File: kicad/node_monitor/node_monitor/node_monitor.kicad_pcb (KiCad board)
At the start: 2 copper layers, 232.4 x 170.2 mm, 68 parts, among them J1 Conn_01x02_Male, J2 Conn_01x02_Male, J3 Conn_01x03_Male, J4 RJ45, J5 Conn_01x02_Male, J6 Conn_01x03_Male, J7 Conn_01x03_Male, J8 Conn_01x02_Male, SW1 SW_DIP_x06

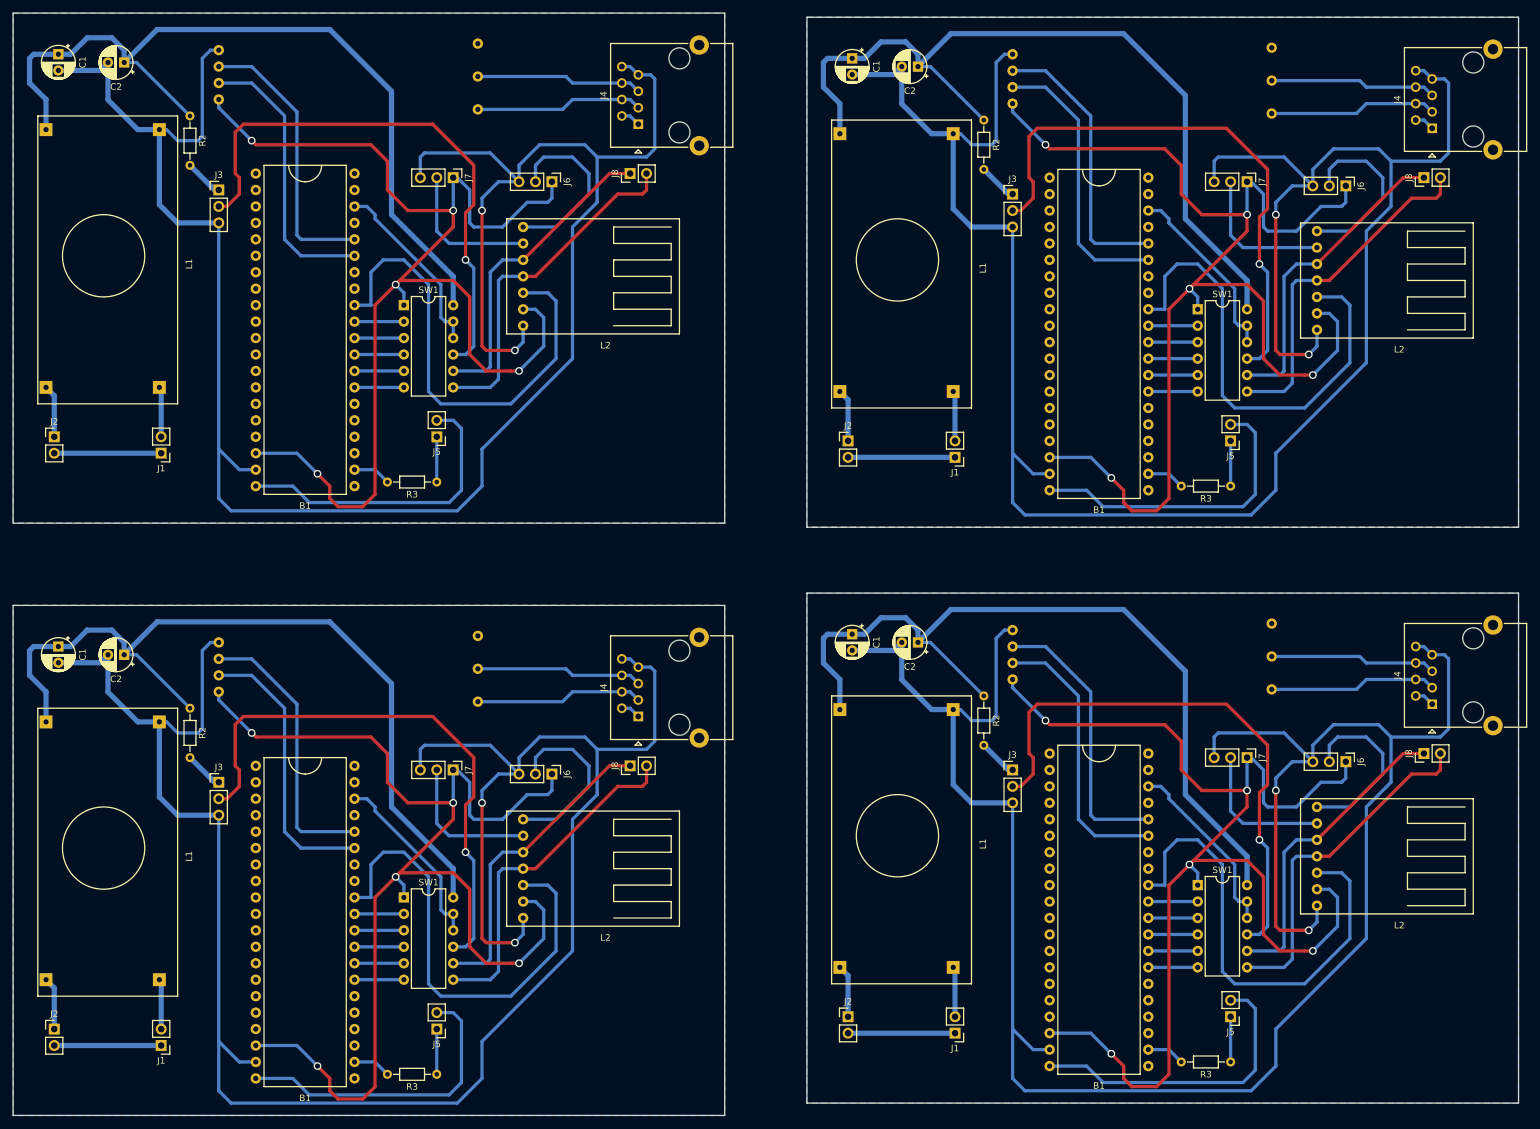
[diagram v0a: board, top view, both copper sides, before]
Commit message: 984
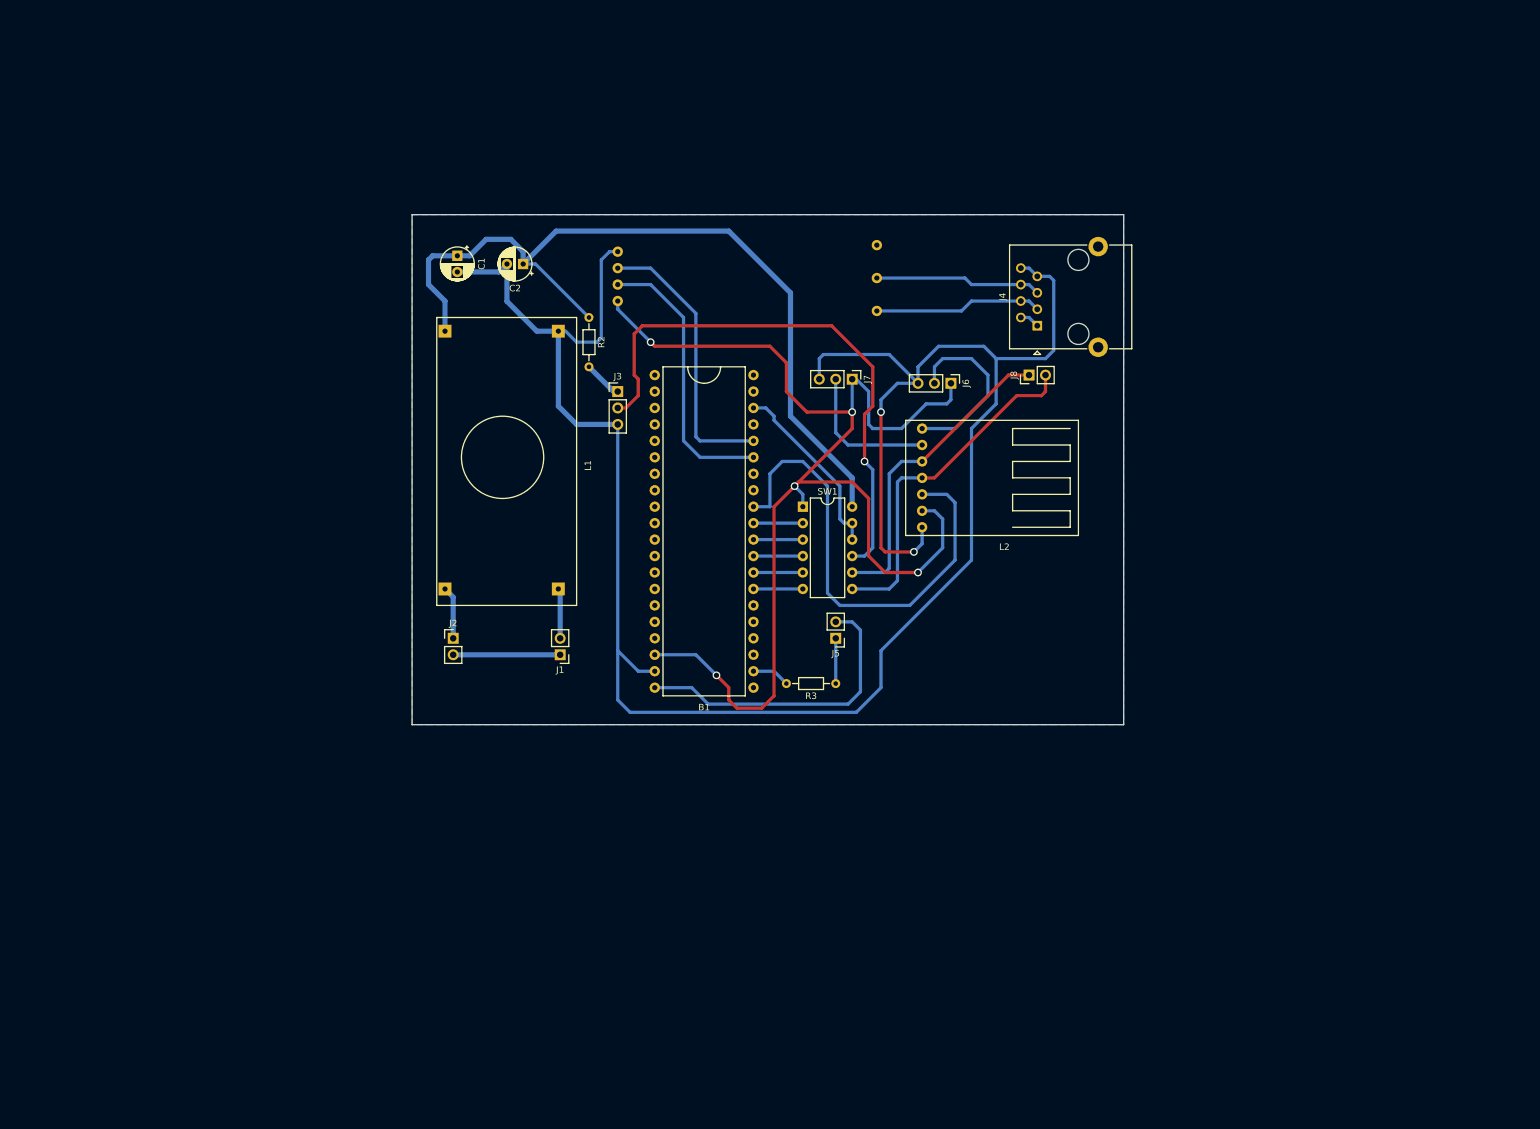
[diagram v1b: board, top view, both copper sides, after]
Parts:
- removed the B1 at (196.2, 138.4)
- removed the B1 at (73.7, 140.3)
- removed the B1 at (196.2, 49.5)
- removed the C1 at (158.1, 114.9)
- removed the C1 at (35.6, 116.8)
- removed the C1 at (158.1, 26.0)
- removed the C2 at (168.3, 116.2)
- removed the C2 at (45.7, 118.1)
- removed the C2 at (168.3, 27.3)
- removed the J1 at (174.0, 176.5)
- removed the J1 at (51.4, 178.4)
- removed the J1 at (174.0, 87.6)
- removed the J2 at (157.5, 174.0)
- removed the J2 at (34.9, 175.9)
- removed the J2 at (157.5, 85.1)
- removed the J3 at (182.9, 135.9)
- removed the J3 at (60.3, 137.8)
- removed the J3 at (182.9, 47.0)
- removed the J4 at (247.7, 125.7)
- removed the J4 at (125.1, 127.6)
- removed the J4 at (247.7, 36.8)
- removed the J5 at (216.5, 174.0)
- removed the J5 at (94.0, 175.9)
- removed the J5 at (216.5, 85.1)
- removed the J6 at (234.3, 134.6)
- removed the J6 at (111.8, 136.5)
- removed the J6 at (234.3, 45.7)
- removed the J7 at (219.1, 134.0)
- removed the J7 at (96.5, 135.9)
- removed the J7 at (219.1, 45.1)
- removed the J8 at (246.4, 133.3)
- removed the J8 at (123.8, 135.3)
- removed the J8 at (246.4, 44.5)
- removed the L1 at (160.0, 153.7)
- removed the L1 at (37.5, 155.6)
- removed the L1 at (160.0, 64.8)
- removed the L2 at (240.0, 146.7)
- removed the L2 at (117.5, 148.6)
- removed the L2 at (240.0, 57.8)
- removed the R1 at (205.7, 116.8)
- removed the R1 at (83.2, 118.7)
- removed the R1 at (205.7, 27.9)
- removed the R2 at (178.4, 124.5)
- removed the R2 at (55.9, 126.4)
- removed the R2 at (178.4, 35.6)
- removed the R3 at (216.5, 181.0)
- removed the R3 at (94.0, 182.9)
- removed the R3 at (216.5, 92.1)
- removed the SW1 at (211.5, 153.7)
- removed the SW1 at (88.9, 155.6)
- removed the SW1 at (211.5, 64.8)
- moved B1 69.0 mm to (135.3, 80.0)
- moved C1 69.0 mm to (97.2, 56.5)
- moved J3 69.0 mm to (121.9, 77.5)
- moved J4 69.0 mm to (186.7, 67.3)
- moved J7 69.0 mm to (158.1, 75.6)
- moved L2 69.0 mm to (179.1, 88.3)
- moved R1 69.0 mm to (144.8, 58.4)
- moved C2 69.0 mm to (107.3, 57.8)
- moved J1 69.0 mm to (113.0, 118.1)
- moved J2 69.0 mm to (96.5, 115.6)
- moved L1 69.0 mm to (99.1, 95.2)
- moved R2 69.0 mm to (117.5, 66.0)
- moved SW1 69.0 mm to (150.5, 95.2)
- moved J5 69.0 mm to (155.6, 115.6)
- moved J6 69.0 mm to (173.4, 76.2)
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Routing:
- net GND1: track 1287.1 -> 321.8 mm, vias 8 -> 2
- net VCCI: track 790.3 -> 197.6 mm, vias 20 -> 5
- net VCCO: track 514.1 -> 128.5 mm
- net RLD: track 345.7 -> 86.4 mm, vias 4 -> 1
- net 3V3: track 303.8 -> 75.9 mm
- net AUX: track 293.0 -> 73.3 mm
- net LTXD: track 215.8 -> 53.9 mm
- net LRXD: track 193.9 -> 48.5 mm
- net RRXD: track 172.6 -> 43.2 mm
- net RTXD: track 172.6 -> 43.2 mm
- net M0: track 111.2 -> 27.8 mm
- net A: track 103.7 -> 25.9 mm
- net B: track 102.9 -> 25.7 mm
- net M1: track 89.5 -> 22.4 mm
- net Net-(J1-Pad1): track 66.0 -> 16.5 mm
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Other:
- board size 232.4 x 170.2 mm -> 109.9 x 78.7 mm
